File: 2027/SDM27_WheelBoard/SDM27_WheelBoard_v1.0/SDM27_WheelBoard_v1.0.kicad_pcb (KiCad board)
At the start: 4 copper layers, 35.5 x 22 mm, 87 parts, among them IC1 TPS2121RUXR, IC2 TPS542951RSAR, IC3 TPS2121RUXR, IC4 MLX90614ESF-BAA-000-SP, IC5 SN74LVC1G17YZPR, IC6 ESP32-C5HF4, IC8 TCAN3403DRBRQ1, J1 WEIPU SA12 7PIN, J2 WEIPU SA6 5Pin, U2 USBLC6-2SC6, Y2 CX1612DB48000D0FPJC1

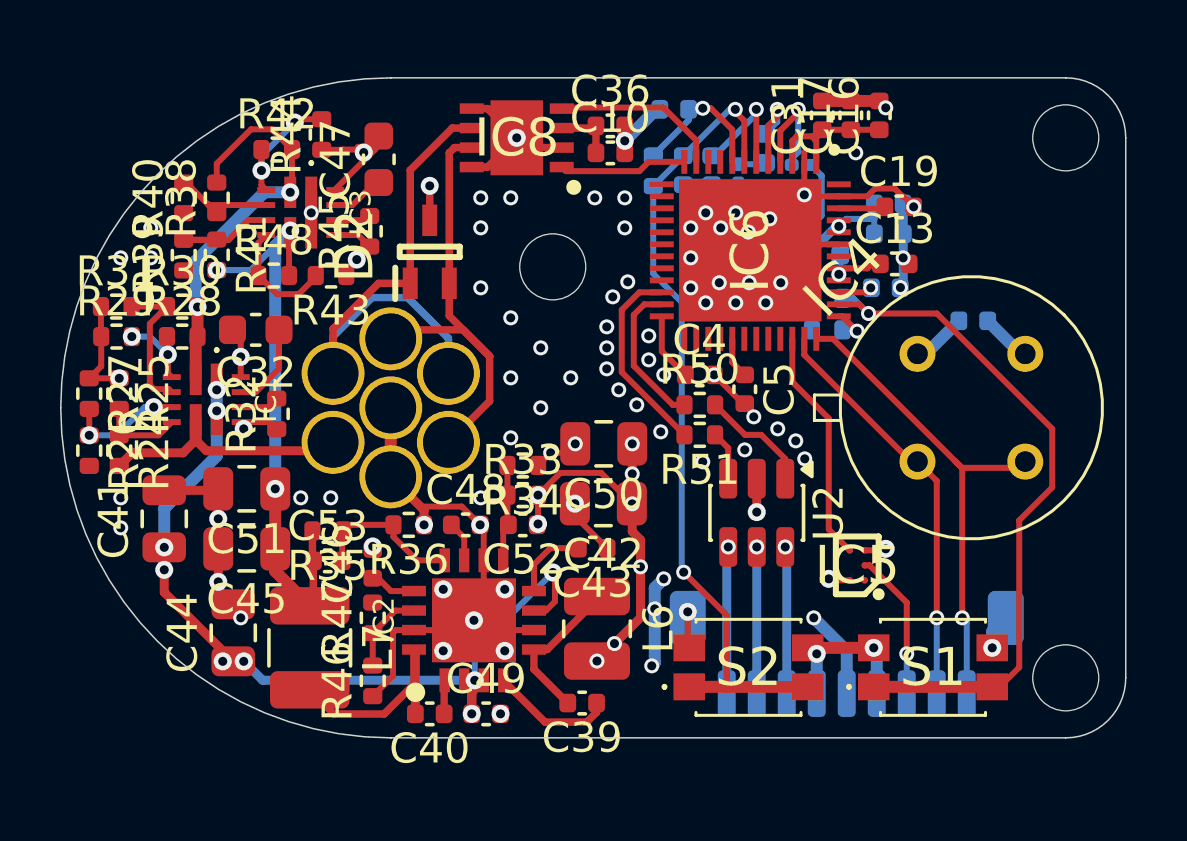
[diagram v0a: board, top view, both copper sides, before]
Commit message: A few more WB edits before bed
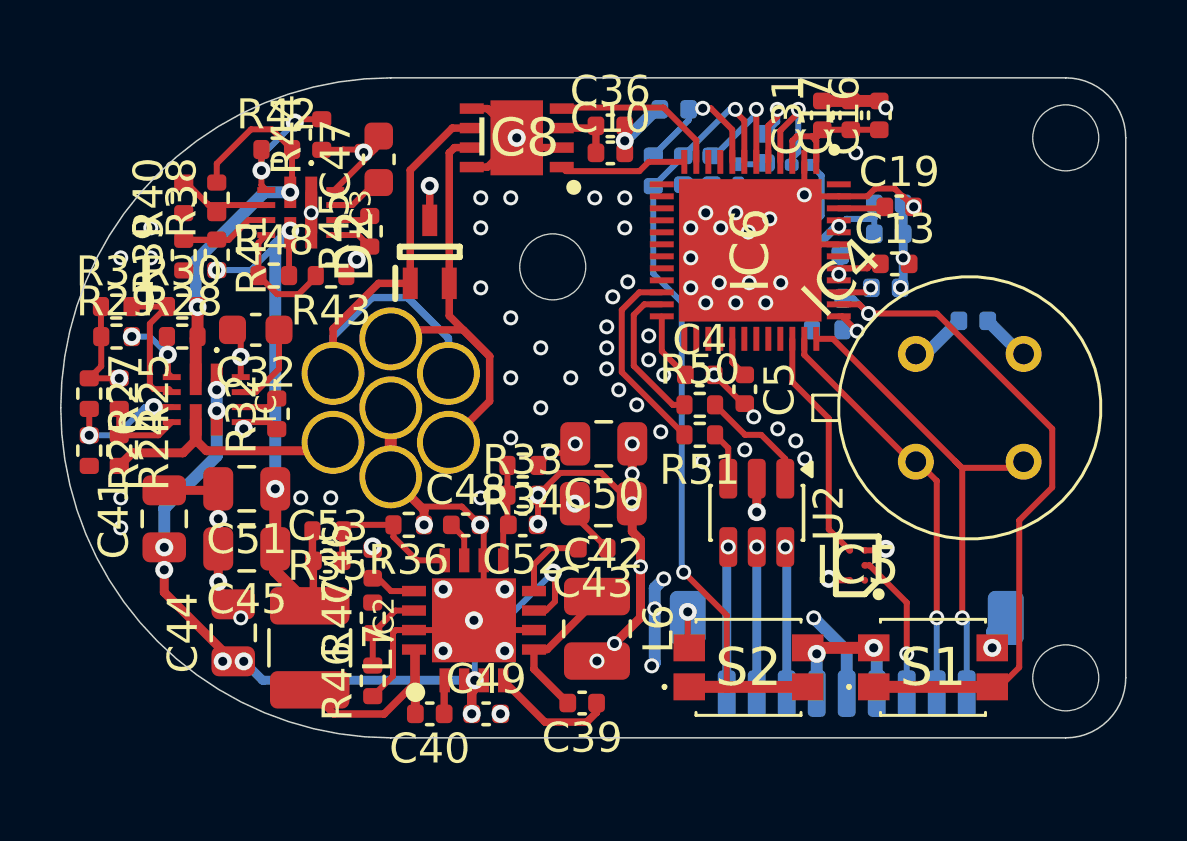
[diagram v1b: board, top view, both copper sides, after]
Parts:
- moved IC4 2.50 mm to (130.3, 100.0)
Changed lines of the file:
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@@
 	(footprint "SDM_Misc:MLX90614ESFBAA000SP"
 		(layer "F.Cu")
-		(at 128.557897 101.792105 45)
+		(at 130.3 100 45)
 		(descr "MLX90614ESF-BAA-000-SP")
 		(tags "Integrated Circuit")
-		(property "Reference" "IC4"
-			(at 2.6 -6.1 45)
-			(layer "F.SilkS")
-			(effects
-				(font
-					(size 1.27 1.27)
-					(thickness 0.254)
-				)
-			)
-		)
 		(property "Value" "MLX90614ESF-BAA-000-SP"
 			(at 2.54 0 45)
@@
 			)
 		)
-		(sheetname "/")
-		(sheetfile "SDM27_WheelBoard_v1.0.kicad_sch")
-		(units
-			(unit
-				(name "A")
-				(pins "2" "1" "3" "4")
+		(property "Reference" "IC4"
+			(at 0.06 -6.1 45)
+			(layer "F.SilkS")
+			(effects
+				(font
+					(size 1.27 1.27)
+					(thickness 0.254)
+				)
 			)
 		)
+		(sheetname "/")
+		(sheetfile "SDM27_WheelBoard_v1.0.kicad_sch")
 		(attr through_hole)
 		(duplicate_pad_numbers_are_jumpers no)
 		(fp_line
-			(start -0.86 -4)
-			(end -1.46 -3.4)
+			(start -3.4 -4)
+			(end -4 -3.4)
 			(stroke
 				(width 0.1)
@@
 		)
 		(fp_line
-			(start -1.46 -3.4)
-			(end -0.860001 -2.799998)
+			(start -4 -3.4)
+			(end -3.400001 -2.799998)
 			(stroke
 				(width 0.1)
@@
 		)
 		(fp_line
-			(start -0.259999 -3.400001)
-			(end -0.86 -4)
+			(start -2.799999 -3.400001)
+			(end -3.4 -4)
 			(stroke
 				(width 0.1)
@@
 		)
 		(fp_line
-			(start -1.833 0.000001)
-			(end -1.833 0.000001)
+			(start -4.373 0.000001)
+			(end -4.373 0.000001)
 			(stroke
 				(width 0.1)
@@
 		)
 		(fp_line
-			(start 6.913 0)
-			(end 6.913 0)
+			(start 4.373 0)
+			(end 4.373 0)
 			(stroke
 				(width 0.1)
@@
 		)
 		(fp_arc
-			(start -1.833 0.000001)
-			(mid 2.54 -4.372997)
-			(end 6.913 0)
+			(start -4.373 0.000001)
+			(mid -0.000001 -4.372998)
+			(end 4.373 0)
 			(stroke
 				(width 0.1)
@@
 		)
 		(fp_arc
-			(start 6.913 0)
-			(mid 2.540002 4.373002)
-			(end -1.833 0.000001)
+			(start 4.373 0)
+			(mid 0.000001 4.373002)
+			(end -4.373 0.000001)
 			(stroke
 				(width 0.1)
@@
 		)
 		(fp_circle
-			(center 2.600001 0)
-			(end 2.600001 -5.400001)
+			(center 0.060001 0)
+			(end 0.060001 -5.400001)
 			(stroke
 				(width 0.05)
@@
 		)
 		(fp_line
-			(start -0.86 -4)
-			(end -0.259999 -3.400001)
+			(start -3.4 -4)
+			(end -2.799999 -3.400001)
 			(stroke
 				(width 0.2)
@@
 		)
 		(fp_line
-			(start -1.46 -3.4)
-			(end -0.86 -4)
+			(start -4 -3.4)
+			(end -3.4 -4)
 			(stroke
 				(width 0.2)
@@
 		)
 		(fp_line
-			(start -0.860001 -2.799998)
-			(end -1.46 -3.4)
+			(start -3.400001 -2.799998)
+			(end -4 -3.4)
 			(stroke
 				(width 0.2)
@@
 		)
 		(fp_line
-			(start -1.833 0.000001)
-			(end -1.833 0.000001)
+			(start -4.373 0.000001)
+			(end -4.373 0.000001)
 			(stroke
 				(width 0.2)
@@
 		)
 		(fp_line
-			(start 6.913 0)
-			(end 6.913 0)
+			(start 4.373 0)
+			(end 4.373 0)
 			(stroke
 				(width 0.2)
@@
 		)
 		(fp_arc
-			(start -1.833 0.000001)
-			(mid 2.54 -4.372997)
-			(end 6.913 0)
+			(start -4.373 0.000001)
+			(mid -0.000001 -4.372998)
+			(end 4.373 0)
 			(stroke
 				(width 0.2)
@@
 		)
 		(fp_arc
-			(start 6.913 0)
-			(mid 2.540002 4.373002)
-			(end -1.833 0.000001)
+			(start 4.373 0)
+			(mid 0.000001 4.373002)
+			(end -4.373 0.000001)
 			(stroke
 				(width 0.2)
@@
 		)
 		(pad "1" thru_hole circle
-			(at 0 0 45)
+			(at -2.54 0 45)
 			(size 1.2 1.2)
 			(drill 0.69)
@@
 		)
 		(pad "2" thru_hole circle
-			(at 2.54 2.54 45)
+			(at 0 2.54 45)
 			(size 1.2 1.2)
 			(drill 0.69)
@@
 		)
 		(pad "3" thru_hole circle
-			(at 5.080002 -0.000001 45)
+			(at 2.540002 -0.000001 45)
 			(size 1.2 1.2)
 			(drill 0.69)
@@
 		)
 		(pad "4" thru_hole circle
-			(at 2.54 -2.54 45)
+			(at 0 -2.54 45)
 			(size 1.2 1.2)
 			(drill 0.69)
@@
 		(layer "Edge.Cuts")
 	)
+	(dimension
+		(type orthogonal)
+		(layer "Edge.Cuts")
+		(pts
+			(xy 131 89) (xy 130.999999 111)
+		)
+		(height 8)
+		(orientation 1)
+		(format
+			(prefix "")
+			(suffix "")
+			(units 3)
+			(units_format 0)
+			(precision 4)
+			(suppress_zeroes yes)
+		)
+		(style
+			(thickness 0.05)
+			(arrow_length 1.27)
+			(text_position_mode 0)
+			(arrow_direction outward)
+			(extension_height 0.58642)
+			(extension_offset 0.5)
+			(keep_text_aligned yes)
+		)
+		(gr_text "22"
+			(at 137.85 100 90)
+			(layer "Edge.Cuts")
+			(effects
+				(font
+					(size 1 1)
+					(thickness 0.15)
+				)
+			)
+		)
+	)
+	(dimension
+		(type orthogonal)
+		(layer "Edge.Cuts")
+		(pts
+			(xy 135.5 94) (xy 100 100.4)
+		)
+		(height -6.5)
+		(orientation 0)
+		(format
+			(prefix "")
+			(suffix "")
+			(units 3)
+			(units_format 0)
+			(precision 4)
+			(suppress_zeroes yes)
+		)
+		(style
+			(thickness 0.05)
+			(arrow_length 1.27)
+			(text_position_mode 0)
+			(arrow_direction outward)
+			(extension_height 0.58642)
+			(extension_offset 0.5)
+			(keep_text_aligned yes)
+		)
+		(gr_text "35.5"
+			(at 117.75 86.35 0)
+			(layer "Edge.Cuts")
+			(effects
+				(font
+					(size 1 1)
+					(thickness 0.15)
+				)
+			)
+		)
+	)
+	(dimension
+		(type orthogonal)
+		(layer "Edge.Cuts")
+		(pts
+			(xy 135 109) (xy 132 109.049999)
+		)
+		(height -1.5)
+		(orientation 0)
+		(format
+			(prefix "")
+			(suffix "")
+			(units 3)
+			(units_format 0)
+			(precision 4)
+			(suppress_zeroes yes)
+		)
+		(style
+			(thickness 0.05)
+			(arrow_length 1.27)
+			(text_position_mode 0)
+			(arrow_direction outward)
+			(extension_height 0.58642)
+			(extension_offset 0.5)
+			(keep_text_aligned yes)
+		)
+		(gr_text "3"
+			(at 133.5 106.35 0)
+			(layer "Edge.Cuts")
+			(effects
+				(font
+					(size 1 1)
+					(thickness 0.15)
+				)
+			)
+		)
+	)
 	(segment
